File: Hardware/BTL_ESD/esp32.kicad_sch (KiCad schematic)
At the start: 11 parts, among them SW3 FLASH, SW4 ENABLE, U5 ESP32-WROOM-32E__4MB_HIGH_TEM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

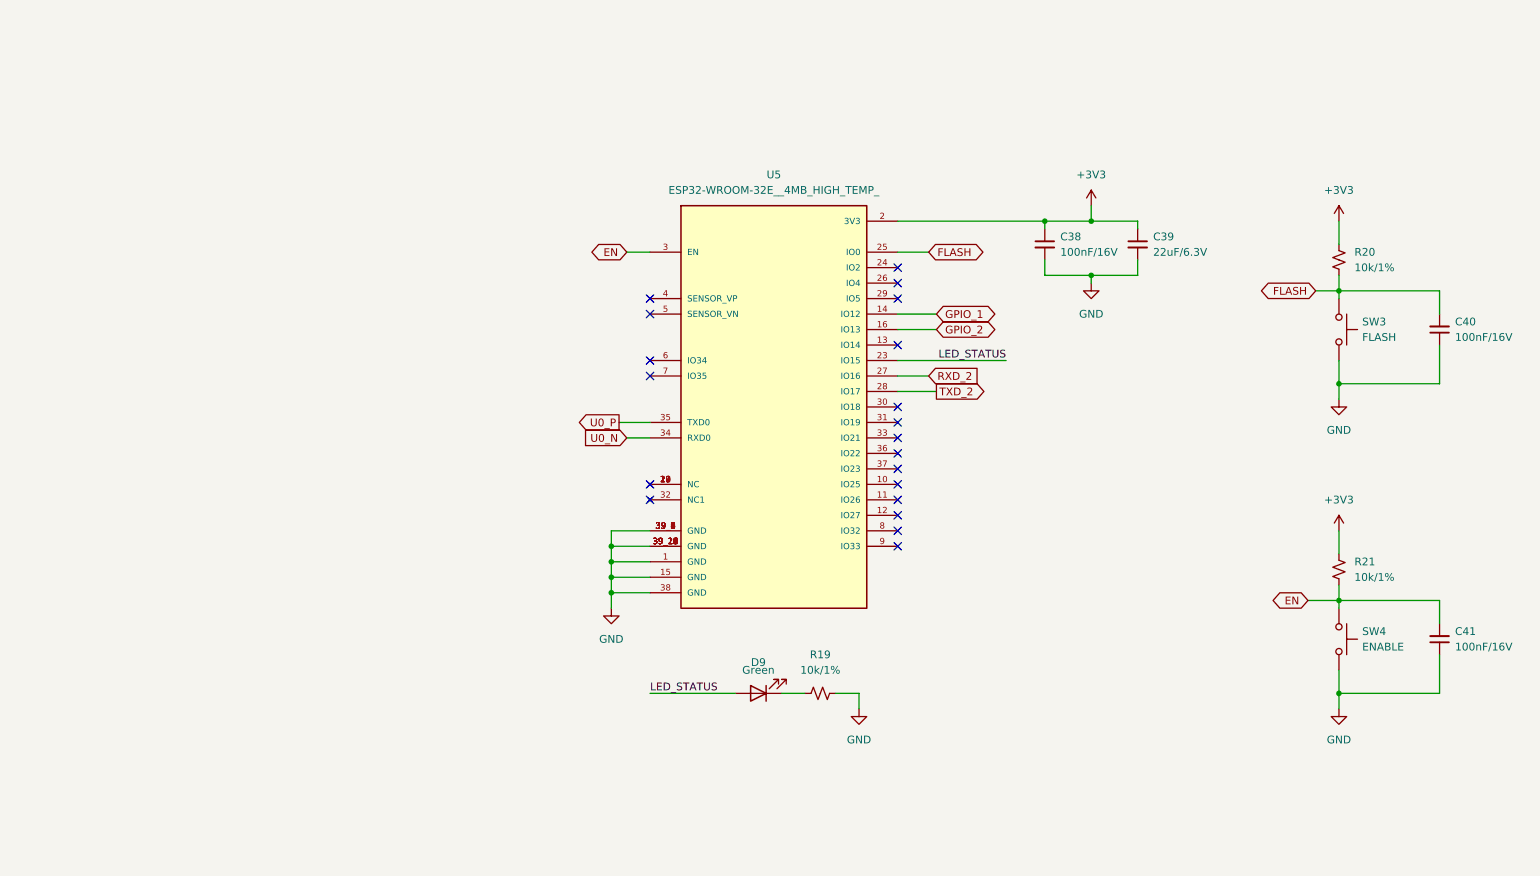
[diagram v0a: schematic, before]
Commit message: update hardware
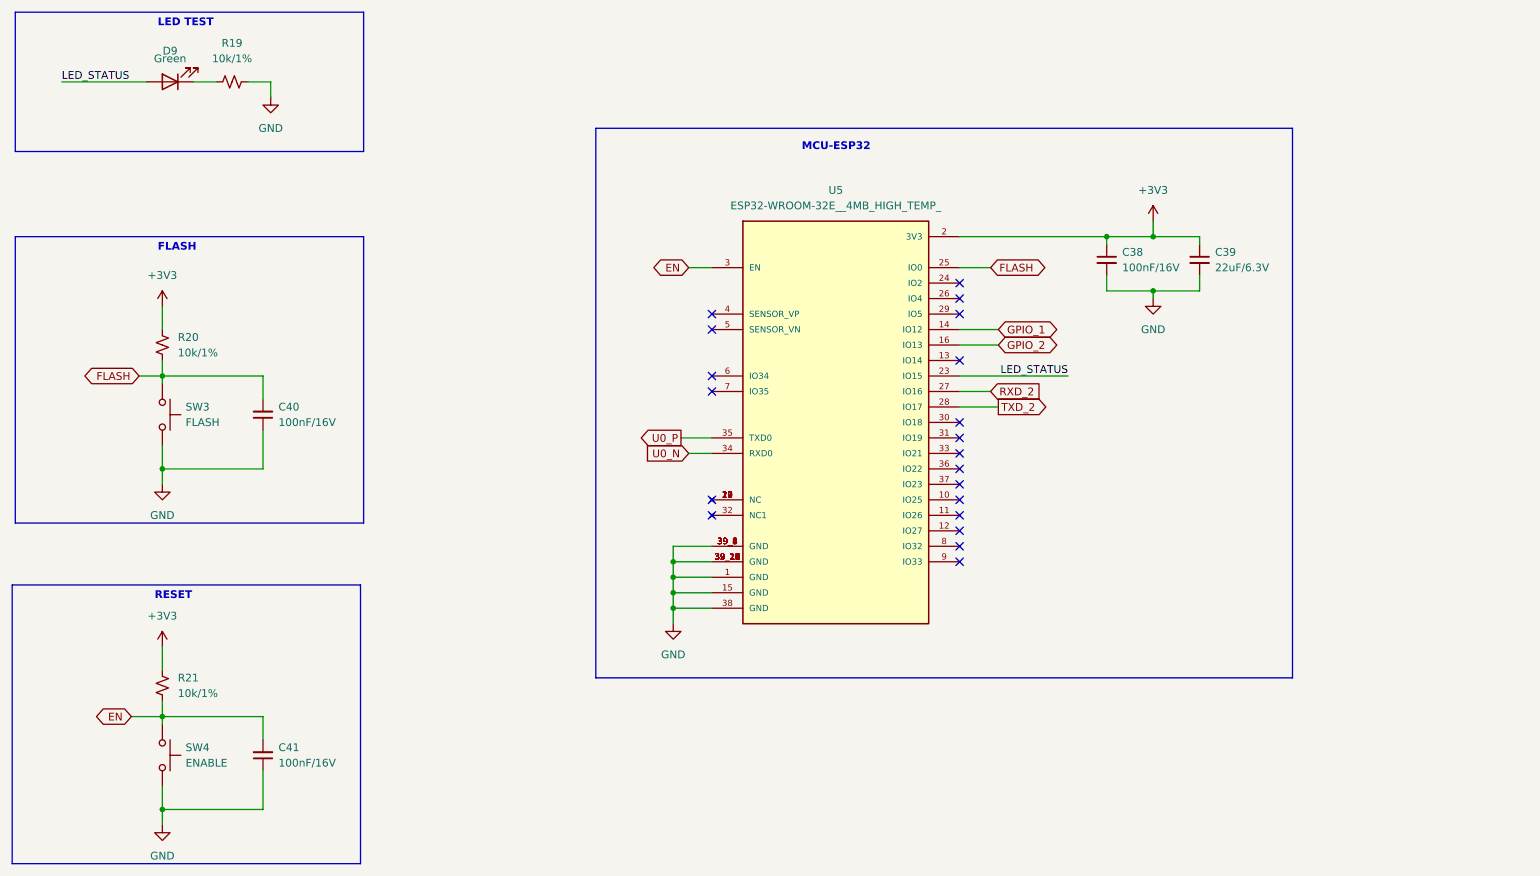
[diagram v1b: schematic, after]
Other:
- note added: "FLASH"
- note added: "LED TEST"
- note added: "MCU-ESP32"
- note added: "RESET"
- moved on the sheet: C38, C39, C40, C41, D9, R19, R20, R21, SW3, SW4, U5
